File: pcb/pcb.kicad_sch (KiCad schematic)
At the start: 15 parts, among them J1 Battery, J2 R_GPIO, J3 L_GPIO, M1 Motor_L, M2 Motor_R, Q12 FS8205A_C2830320, U1 DRV8220SDG, U2 DRV8220SDG, U3 DW01A_C18164398

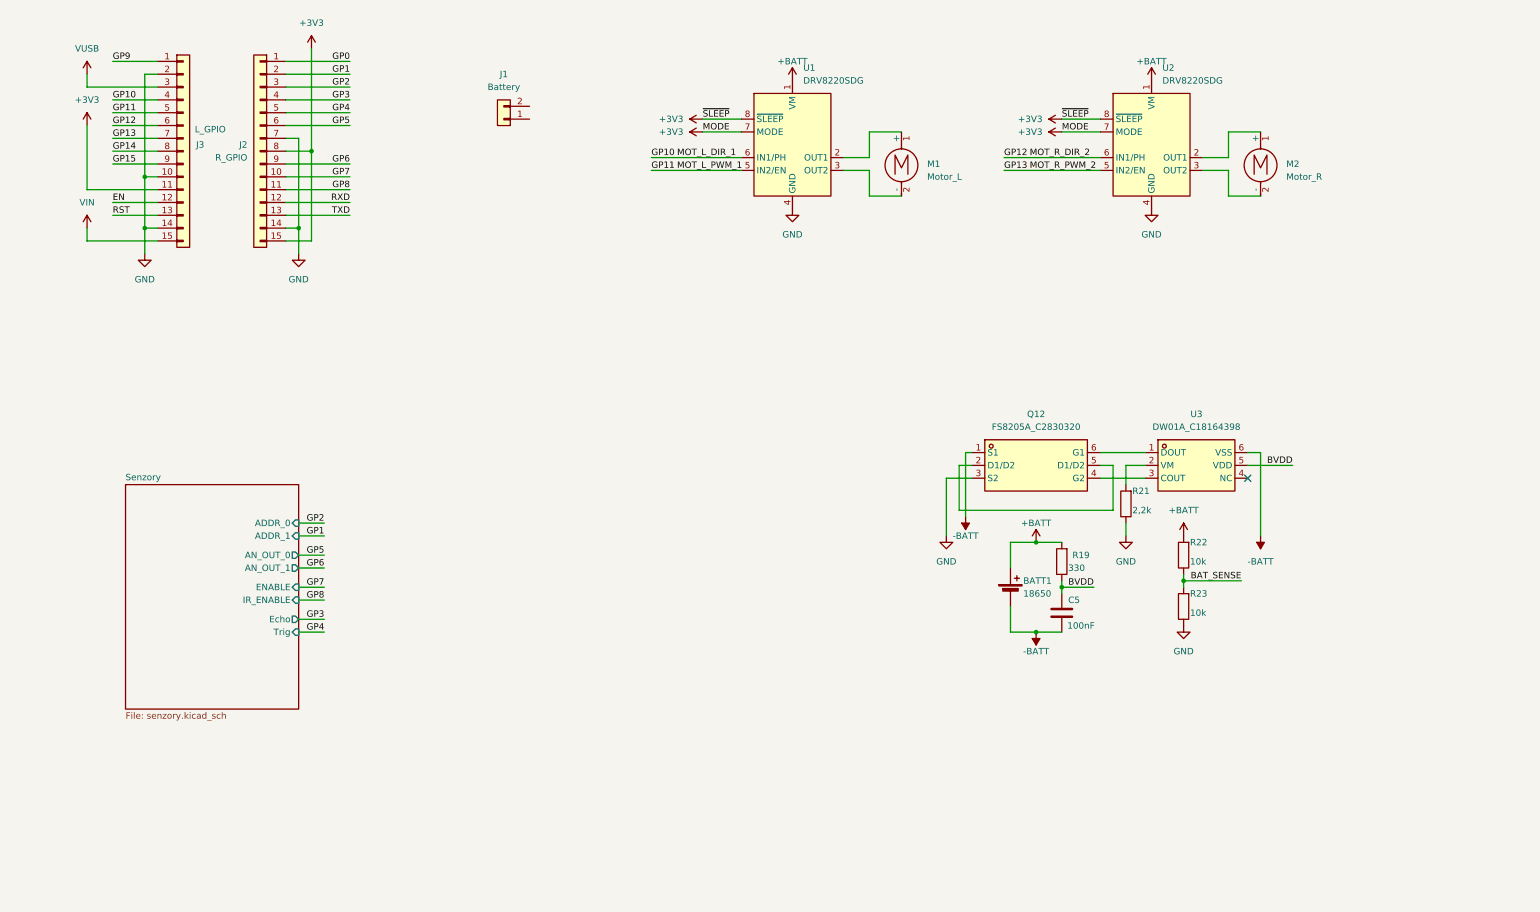
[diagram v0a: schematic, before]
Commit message: schéma
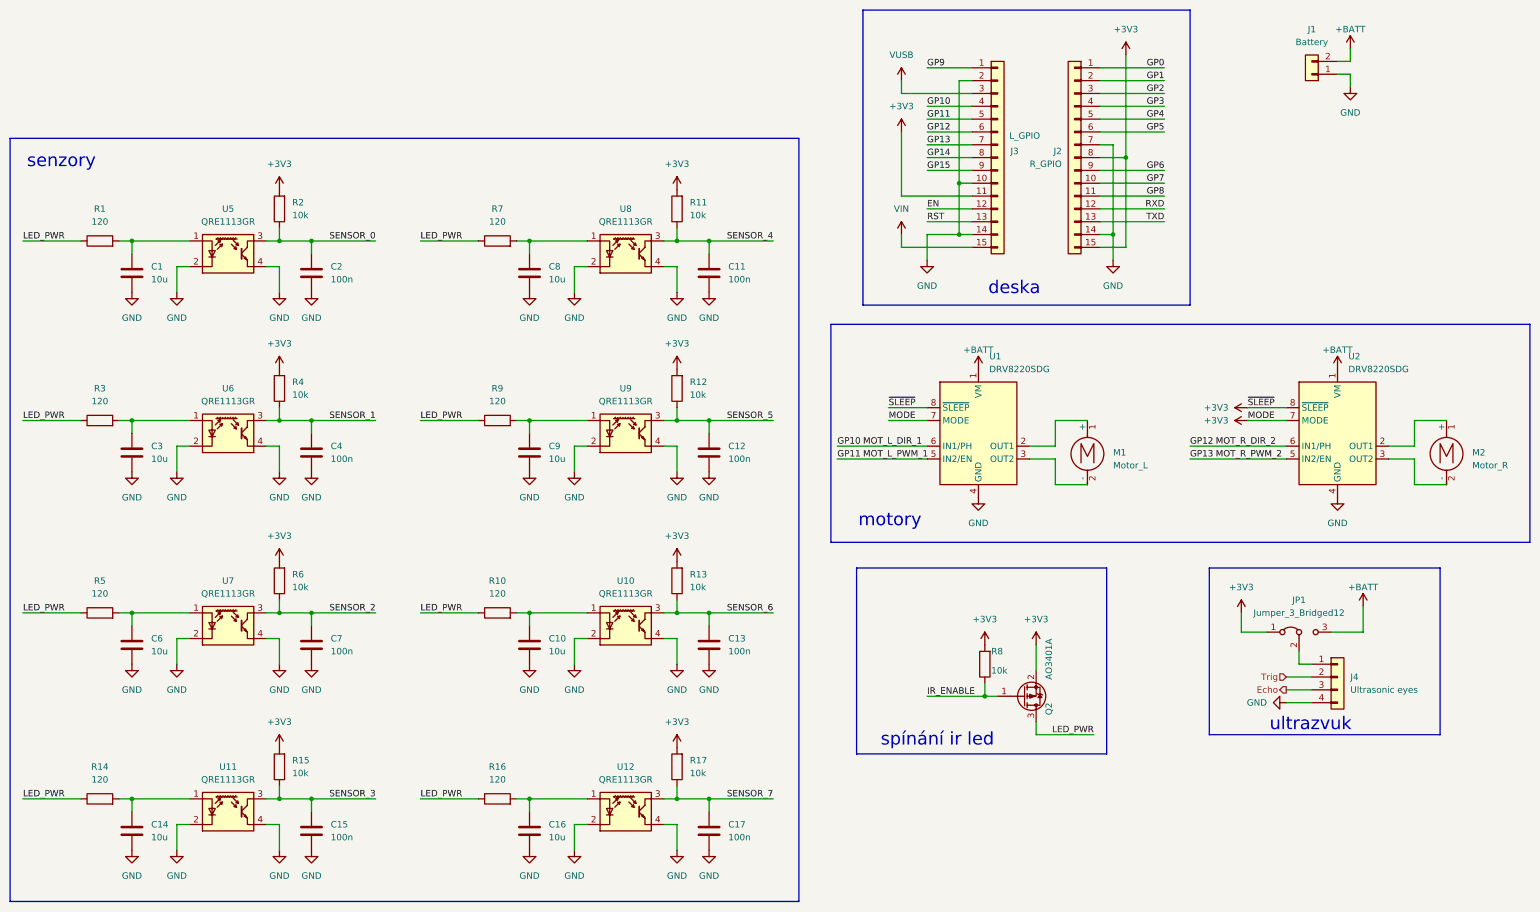
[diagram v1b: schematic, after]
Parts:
- removed BATT1: 18650, easyeda2kicad:BATTERY-SMD_18650-1S-L77.1-W20.7-1, symbol Device:Battery_Cell
- removed C5: 100nF, Capacitor_SMD:C_0603_1608Metric, symbol Device:C
- removed Q12: FS8205A_C2830320, easyeda2kicad:SOT-23-6_L2.9-W1.6-P0.95-LS2.8-BR, symbol easyeda2kicad:FS8205A_C2830320
- removed R19: 330, Resistor_SMD:R_0603_1608Metric, symbol Device:R
- removed R21: 2,2k, Resistor_SMD:R_0603_1608Metric, symbol Device:R
- removed R22, R23: 10k, Resistor_SMD:R_0603_1608Metric, symbol Device:R
- removed U3: DW01A_C18164398, easyeda2kicad:SOT-23-6_L2.9-W1.6-P0.95-LS2.8-BR, symbol easyeda2kicad:DW01A_C18164398
- added C1, C10, C14, C16, C3, C6, C8, C9: 10u, Capacitor_SMD:C_0603_1608Metric_Pad1.08x0.95mm_HandSolder, symbol Device:C
- added C11, C12, C13, C15, C17, C2, C4, C7: 100n, Capacitor_SMD:C_0603_1608Metric_Pad1.08x0.95mm_HandSolder, symbol Device:C
- added J4: Ultrasonic eyes, Connector_PinSocket_2.54mm:PinSocket_1x04_P2.54mm_Vertical, symbol Connector_Generic:Conn_01x04
- added JP1: Jumper_3_Bridged12, Connector_PinHeader_2.54mm:PinHeader_1x03_P2.54mm_Vertical, symbol Jumper:Jumper_3_Bridged12
- added Q2: AO3401A, Package_TO_SOT_SMD:SOT-23, symbol Transistor_FET:AO3401A
- added R1, R10, R14, R16, R3, R5, R7, R9: 120, Resistor_SMD:R_0603_1608Metric_Pad0.98x0.95mm_HandSolder, symbol Device:R
- added R11, R12, R13, R15, R17, R2, R4, R6: 10k, Resistor_SMD:R_0603_1608Metric_Pad0.98x0.95mm_HandSolder, symbol Device:R
- added R8: 10k, Resistor_SMD:R_0603_1608Metric, symbol Device:R
- added U10, U11, U12, U5, U6, U7, U8, U9: QRE1113GR, OptoDevice:OnSemi_CASE100CY, symbol Sensor_Proximity:QRE1113GR
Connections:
- net +3V3: now also JP1.1 (A), Q2.2 (S), R11.2, R12.2, R13.2, R15.2, R17.2, R2.2, R4.2, R6.2, R8.2
- net +BATT: now also J1.2 (Pin_2), JP1.3 (B)
- net GND: now also J1.1 (Pin_1), C1.2, C10.2, C11.2, C12.2, C13.2, C14.2, C15.2, C16.2, C17.2, C2.2, C3.2, C4.2, C6.2, C7.2, C8.2, C9.2, J4.4 (Pin_4), U10.2 (K), U10.4, U11.2 (K), U11.4, U12.2 (K), U12.4, U5.2 (K), U5.4, U6.2 (K), U6.4, U7.2 (K), U7.4, U8.2 (K), U8.4, U9.2 (K), U9.4
- new net: C1.1, R1.2, U5.1 (A)
- new net: C9.1, R9.2, U9.1 (A)
- new net: J4.1 (Pin_1), JP1.2 (C)
- new net: C6.1, R5.2, U7.1 (A)
- new net: C3.1, R3.2, U6.1 (A)
- new net: C16.1, R16.2, U12.1 (A)
- new net: C8.1, R7.2, U8.1 (A)
- new net: C10.1, R10.2, U10.1 (A)
- new net: C14.1, R14.2, U11.1 (A)
- new net Echo: J4.3 (Pin_3)
- new net IR_ENABLE: Q2.1 (G), R8.1
- new net LED_PWR: Q2.3 (D), R1.1, R10.1, R14.1, R16.1, R3.1, R5.1, R7.1, R9.1
- new net SENSOR_0: C2.1, R2.1, U5.3
- new net SENSOR_1: C4.1, R4.1, U6.3
- new net SENSOR_2: C7.1, R6.1, U7.3
- new net SENSOR_3: C15.1, R15.1, U11.3
- new net SENSOR_4: C11.1, R11.1, U8.3
- new net SENSOR_5: C12.1, R12.1, U9.3
- new net SENSOR_6: C13.1, R13.1, U10.3
- new net SENSOR_7: C17.1, R17.1, U12.3
- new net Trig: J4.2 (Pin_2)
- no-connect marks 1 -> 0
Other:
- removed sheet Senzory
- note added: "deska"
- note added: "motory"
- note added: "senzory"
- note added: "spínání ir led"
- note added: "ultrazvuk"
- moved on the sheet: J1, J2, J3, M1, M2, U1, U2
